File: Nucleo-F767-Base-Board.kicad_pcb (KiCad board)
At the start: 2 copper layers, 120 x 130 mm, 81 parts, among them IC1 TLP152, IC2 TLP152, IC3 TLP152, IC4 TLP152, J1 Conn_01x02_Pin, J14 Conn_01x02_Pin, J15 Conn_01x02_Pin, J16 Conn_01x02_Pin, J17 Conn_01x02_Pin, J2 Conn_01x02_Pin, J20 Conn_01x03_Pin, J21 Conn_01x03_Pin, J24 Conn_01x03_Pin, J25 Conn_01x03_Pin, J3 Conn_01x02_Pin, J4 Conn_01x02_Pin, J5 Conn_01x02_Pin, J6 Conn_01x02_Pin, J7 Conn_01x02_Pin, J8 Conn_01x02_Pin, J9 Conn_01x02_Pin, Q1 RS6G120BGTB1, Q2 RS6G120BGTB1, Q3 RS6G120BGTB1, Q4 RS6G120BGTB1, SW1 SW_Push, SW2 SW_Push, U1 MC78M09CDTRKG, U4 TBD62783A, U5 TPS5450, U6 MCP2551-I-P

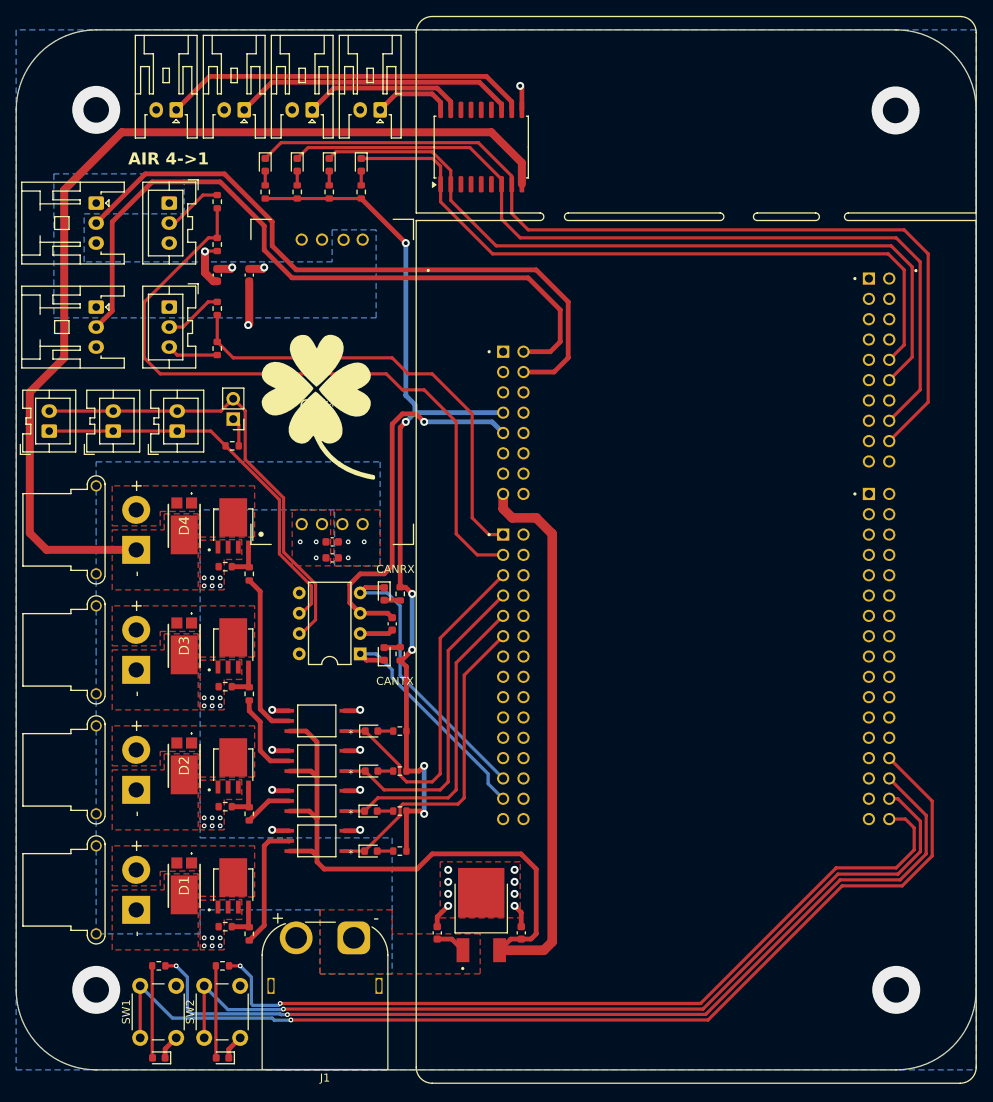
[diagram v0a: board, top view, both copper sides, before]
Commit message: Update.
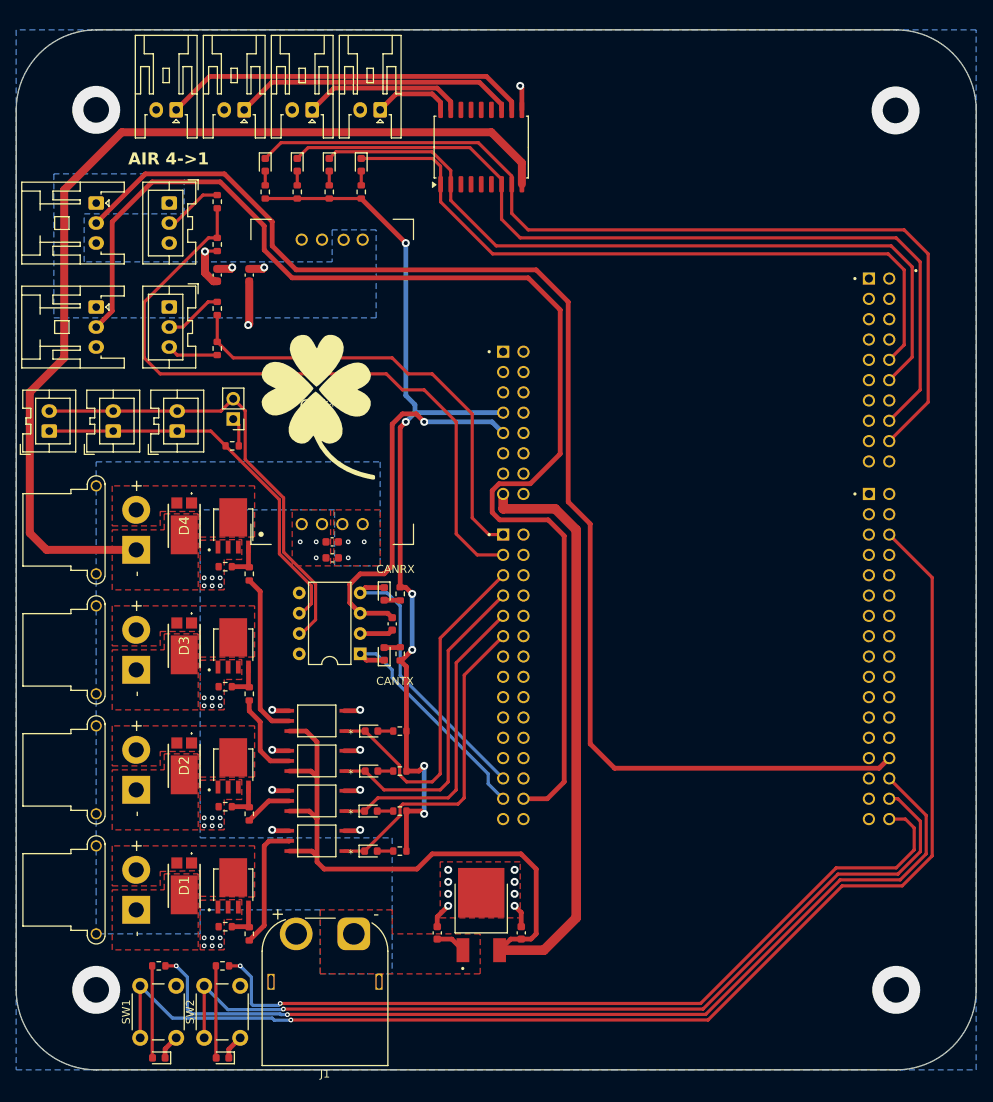
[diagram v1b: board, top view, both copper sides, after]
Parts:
- moved J1 0.50 mm to (72.2, 143.0)
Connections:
- A1 pad CN10_28: SW1 -> PWM1
- A1 pad CN10_6: unconnected-(A1D-D5/TIMER_A_PWM2-PadCN10_6) -> SW1
- A1 pad CN8_2: PWM2 -> unconnected-(A1B-D43/SDMMC_D0-PadCN8_2)
- A1 pad CN8_4: PWM1 -> unconnected-(A1B-D44/SDMMC_D1/I2S_A_CKIN-PadCN8_4)
- A1 pad CN9_28: unconnected-(A1C-D63/SAI_B_FS-PadCN9_28) -> PWM2
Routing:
- net PWM1: track 83.3 -> 165.5 mm
- net PWM2: track 89.5 -> 158.5 mm
- net SW1: track 130.2 -> 158.2 mm
- net +9V: track 140.9 -> 145.4 mm
